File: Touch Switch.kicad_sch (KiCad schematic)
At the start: 51 parts, among them J1 Conn_01x01_Pin, J2 Conn_02x04_Counter_Clockwise, J3 Conn_01x01_Pin, J4 Conn_01x01_Pin, J5 Conn_01x01_Pin, J6 Conn_01x01_Pin, J7 Conn_01x01_Pin, J8 Conn_01x01_Pin, K1 Relay_SPST-NO, K2 Relay_SPST-NO, K3 Relay_SPST-NO, K4 Relay_SPST-NO, Q1 MMBT3904, Q2 MMBT3904, Q3 MMBT3904, Q5 MMBT3904, T1 Transformer_1P_2S, U1 SCJT1117B-3.3-A

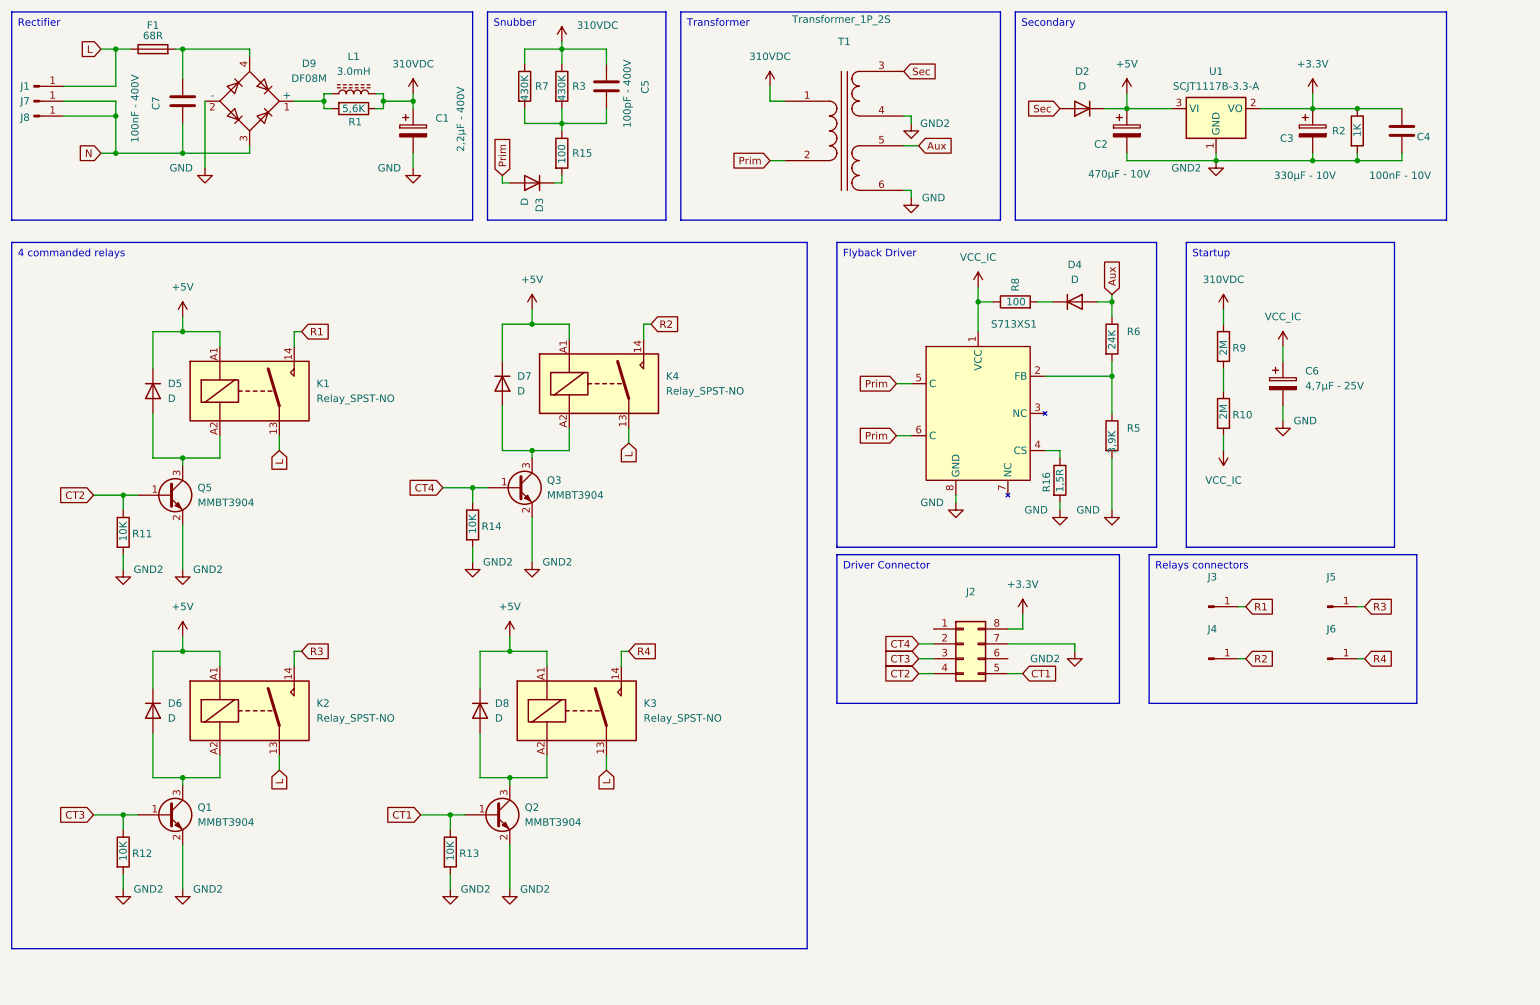
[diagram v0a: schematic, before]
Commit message: PCB V3
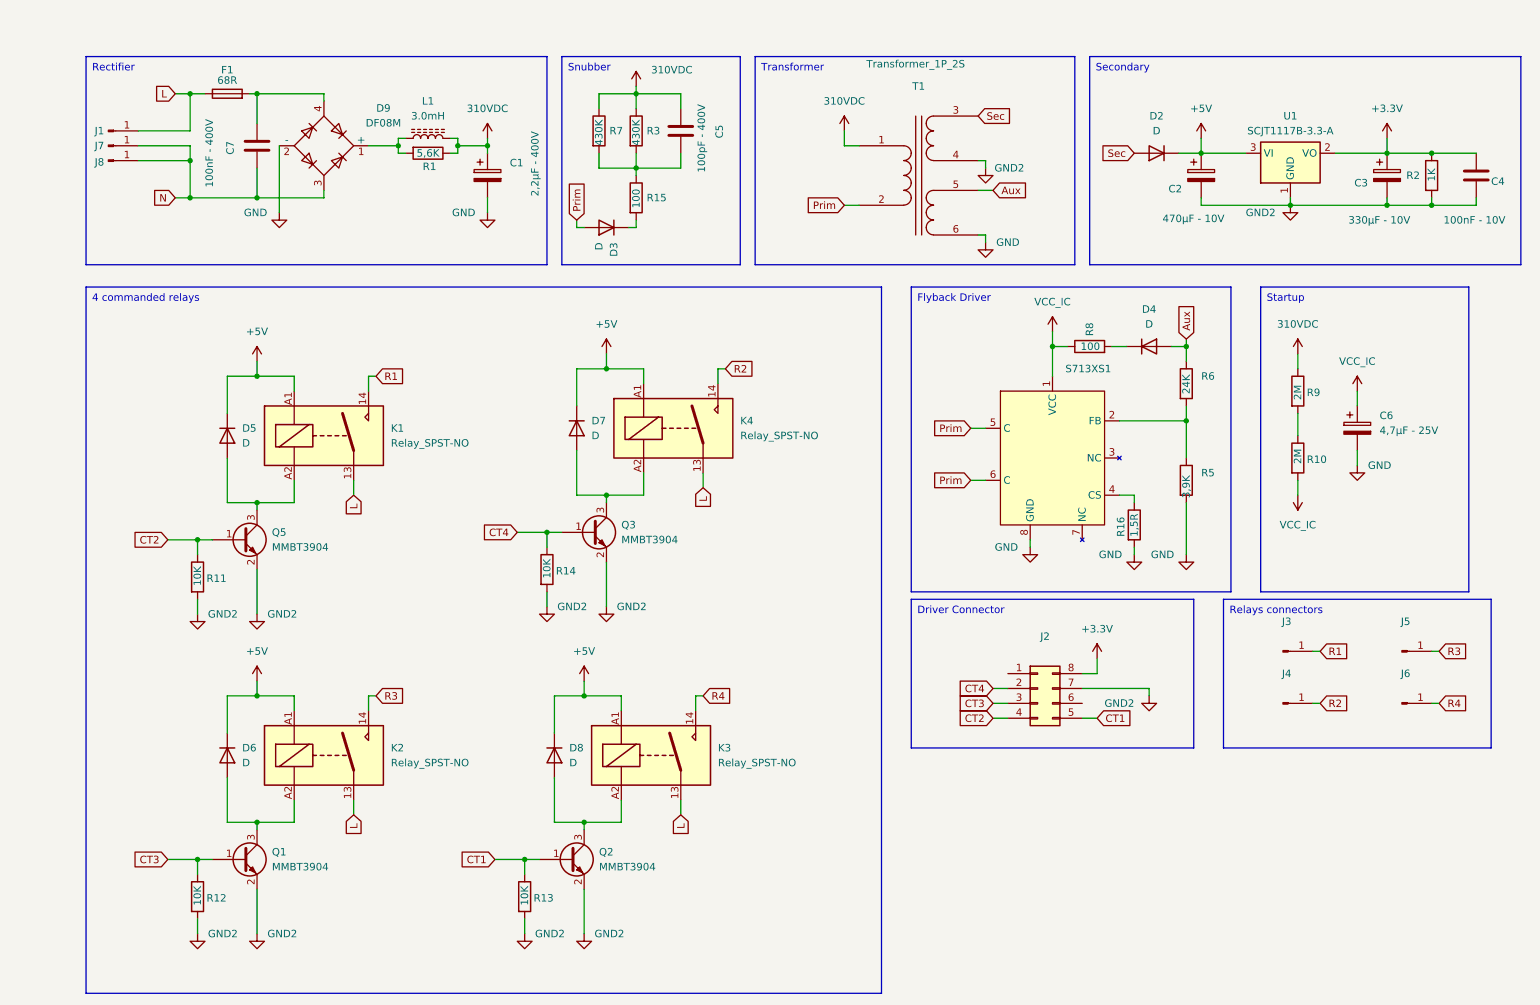
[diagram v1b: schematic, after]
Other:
- moved on the sheet: C1, C2, C3, C4, C5, C6, C7, D2, D3, D4, D5, D6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
